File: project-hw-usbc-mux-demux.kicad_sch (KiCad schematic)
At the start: 0 parts

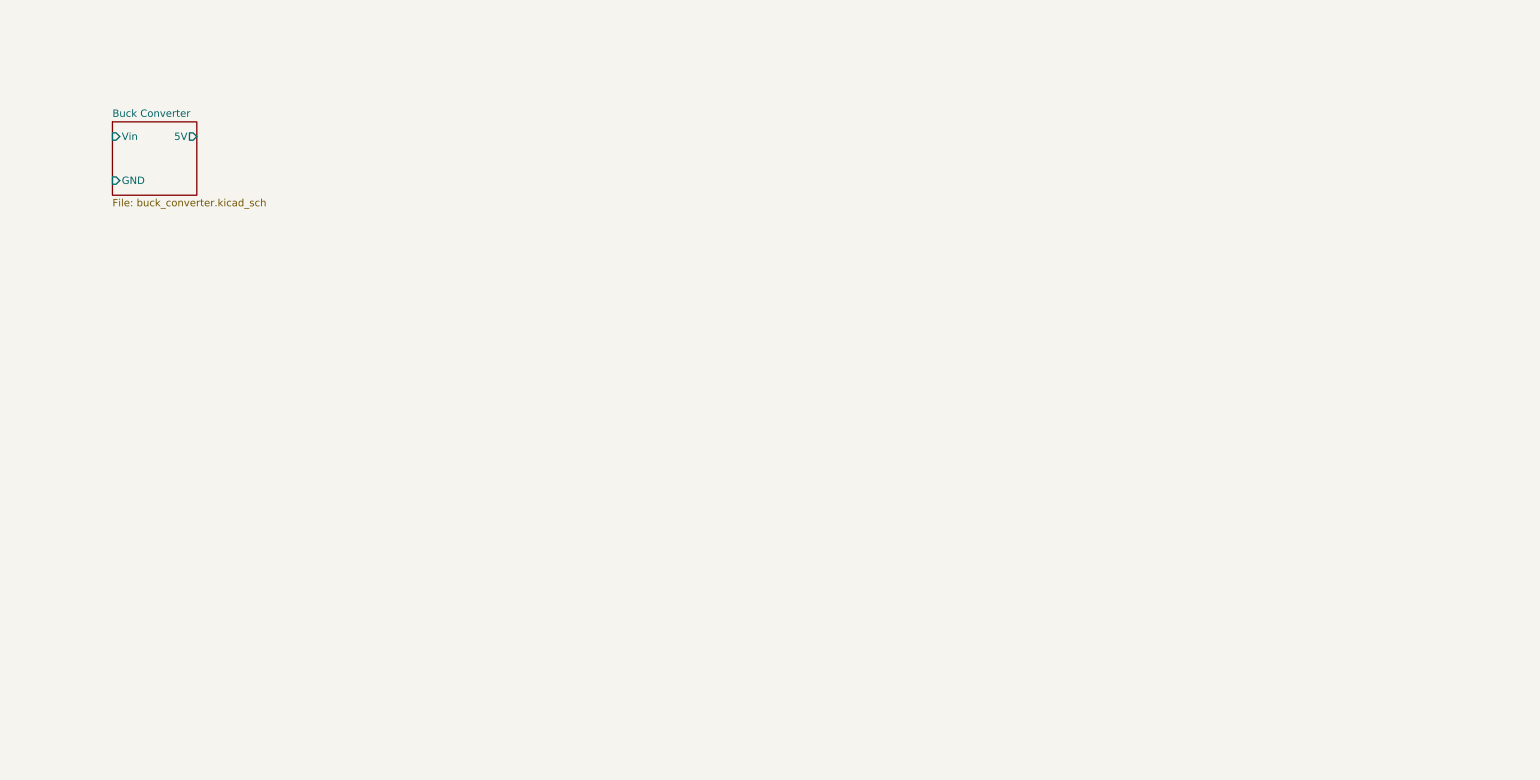
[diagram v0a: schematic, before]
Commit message: sch: first draft
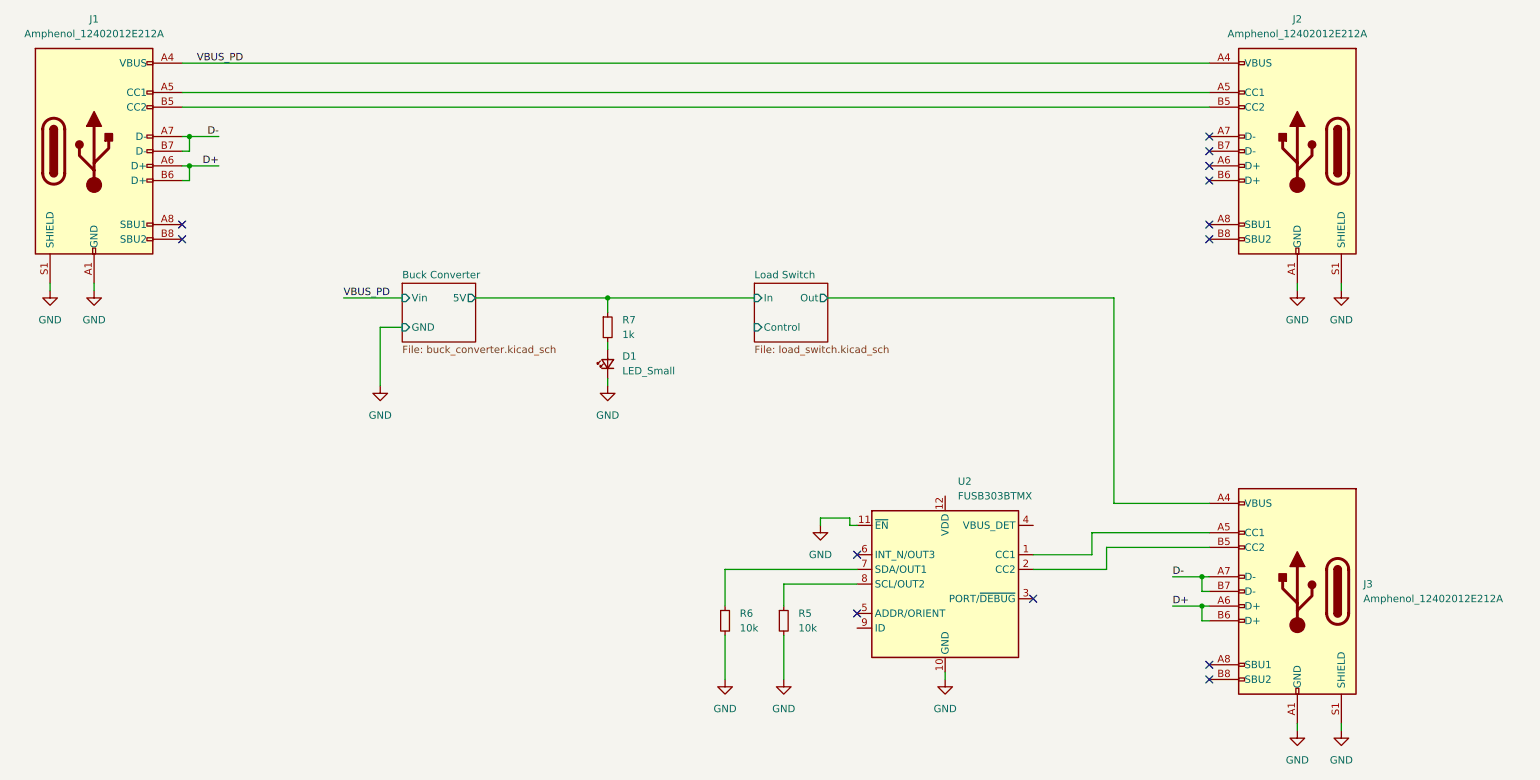
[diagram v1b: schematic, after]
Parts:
- added D1: LED_Small, LED_SMD:LED_0603_1608Metric, symbol Device:LED_Small
- added J1, J2, J3: Amphenol_12402012E212A, symbol Amphenol_12402012E212A:Amphenol_12402012E212A
- added R5, R6: 10k, Resistor_SMD:R_0603_1608Metric, symbol Device:R_Small
- added R7: 1k, Resistor_SMD:R_0603_1608Metric, symbol Device:R_Small
- added U2: FUSB303BTMX, QFN:Texas_X2QFN-12_1.6x1.6mm_P0.4mm, symbol onsemi_FUSB303BTMX:FUSB303BTMX
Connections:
- net Buck Converter/5V: now also R7.1
- new net: R6.1, U2.7 (SDA/OUT1)
- new net: J3.A5 (CC1), U2.1 (CC1)
- new net: J3.B5 (CC2), U2.2 (CC2)
- new net: J1.A5 (CC1), J2.A5 (CC1)
- new net: J1.B5 (CC2), J2.B5 (CC2)
- new net: R5.1, U2.8 (SCL/OUT2)
- new net: D1.2 (A), R7.2
- new net D+: J1.A6 (D+), J1.B6 (D+), J3.A6 (D+), J3.B6 (D+)
- new net D-: J1.A7 (D-), J1.B7 (D-), J3.A7 (D-), J3.B7 (D-)
- new net GND: D1.1 (K), J1.A1 (GND), J1.A12 (GND), J1.B1 (GND), J1.B12 (GND), J1.S1 (SHIELD), J2.A1 (GND), J2.A12 (GND), J2.B1 (GND), J2.B12 (GND), J2.S1 (SHIELD), J3.A1 (GND), J3.A12 (GND), J3.B1 (GND), J3.B12 (GND), J3.S1 (SHIELD), R5.2, R6.2, U2.10 (GND), U2.11 (~{EN})
- new net Load Switch/Out: J3.A4 (VBUS), J3.A9 (VBUS), J3.B4 (VBUS), J3.B9 (VBUS)
- new net VBUS_PD: J1.A4 (VBUS), J1.A9 (VBUS), J1.B4 (VBUS), J1.B9 (VBUS), J2.A4 (VBUS), J2.A9 (VBUS), J2.B4 (VBUS), J2.B9 (VBUS)
- no-connect marks 0 -> 13
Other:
- added sheet Load Switch (load_switch.kicad_sch)
